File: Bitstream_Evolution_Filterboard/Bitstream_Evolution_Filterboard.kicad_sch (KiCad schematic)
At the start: 7 parts, among them J1 Conn_01x15_Female, J2 Conn_01x15_Female, J3 Conn_01x10_Female, J4 Conn_01x10_Female, J5 Conn_01x02_Male

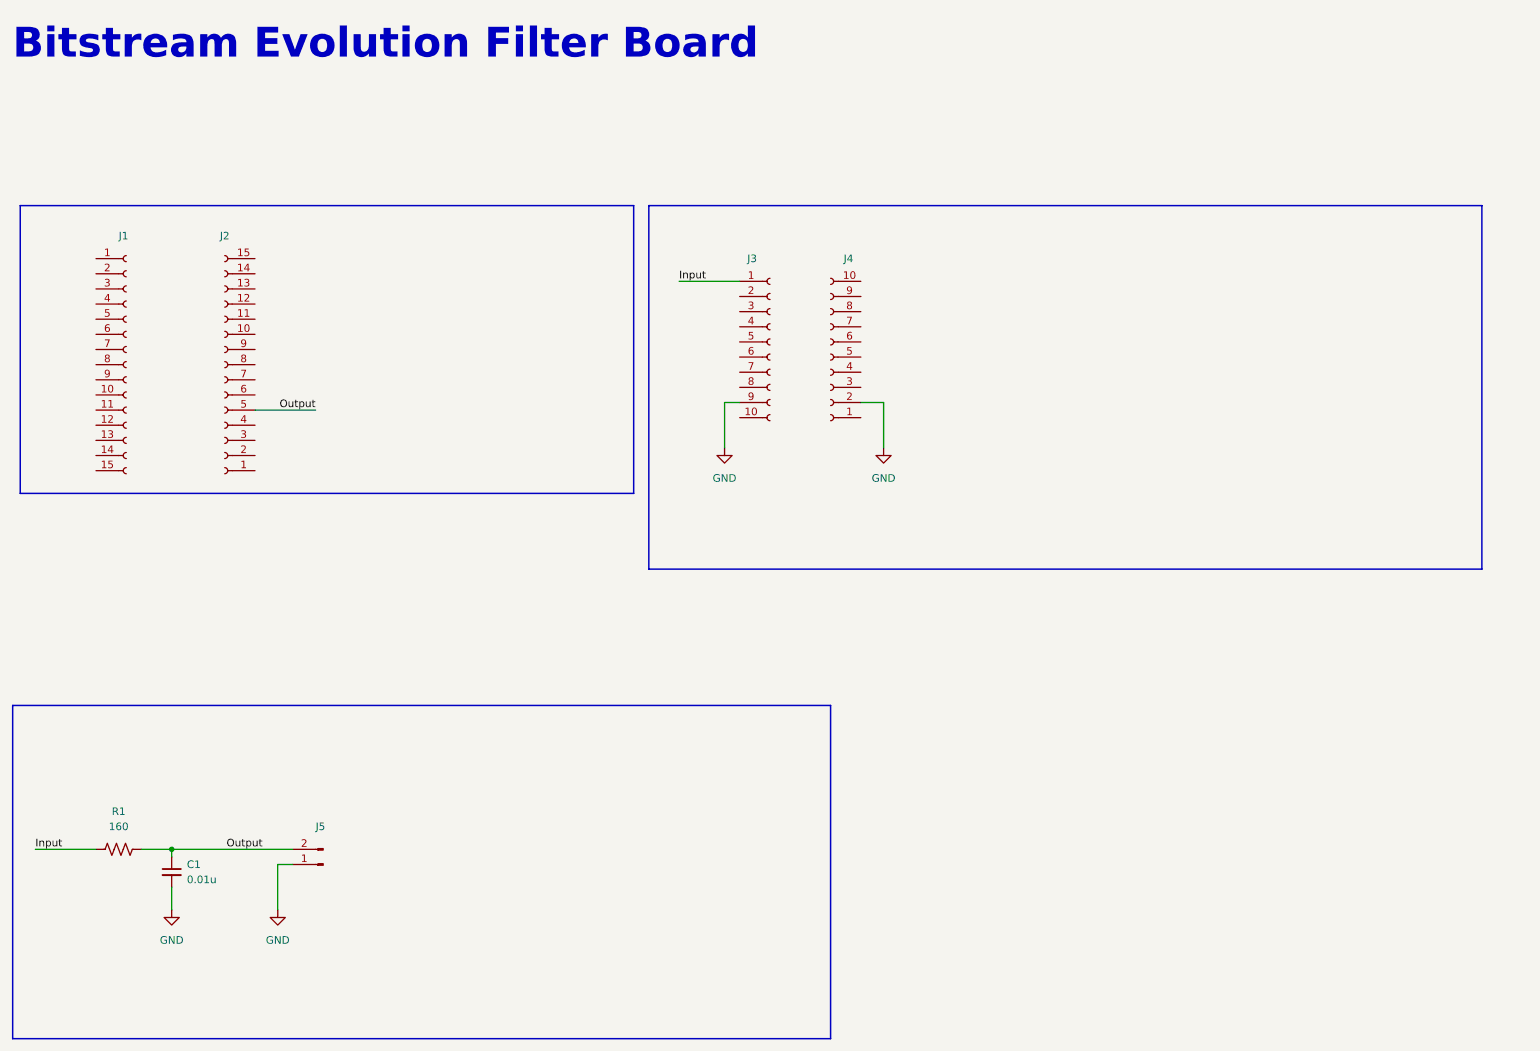
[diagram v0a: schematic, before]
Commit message: Updates to Hardware
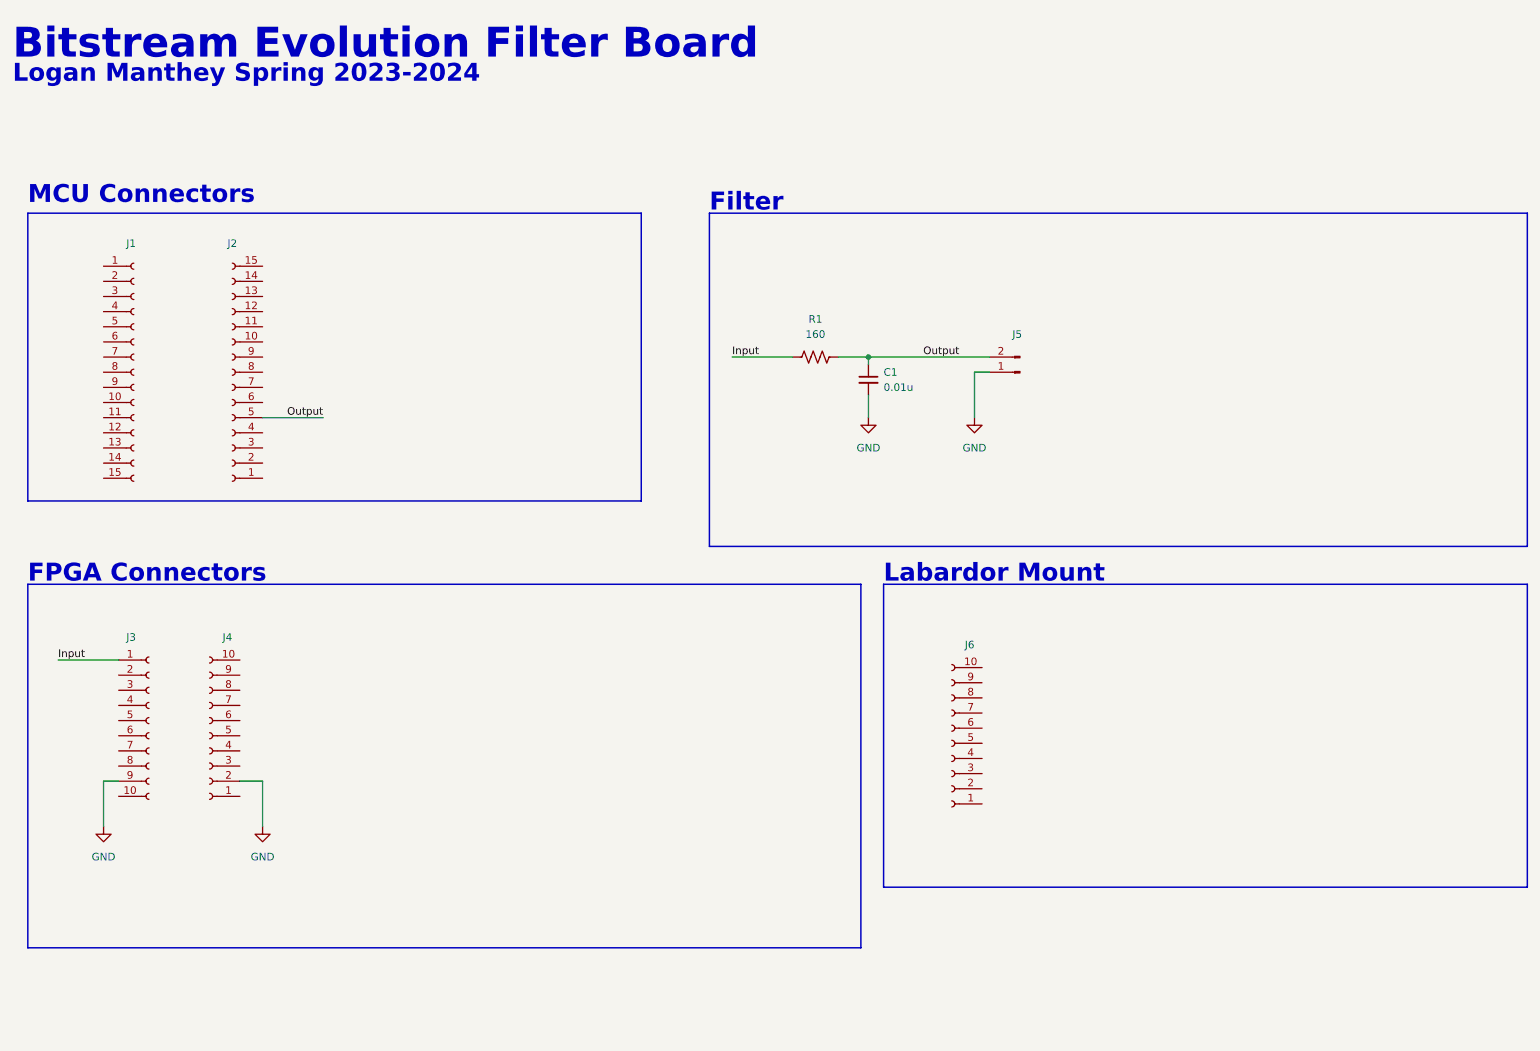
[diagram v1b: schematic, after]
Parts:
- added J6: Conn_01x10_Female, Connector_PinSocket_2.54mm:PinSocket_1x10_P2.54mm_Vertical, symbol Connector:Conn_01x10_Female
- J1, J2: footprint Connector_PinSocket_1.00mm:PinSocket_1x15_P1.00mm_Vertical -> Connector_PinSocket_2.54mm:PinSocket_1x15_P2.54mm_Vertical
- J3, J4: footprint Connector_PinSocket_1.00mm:PinSocket_1x10_P1.00mm_Vertical -> Connector_PinSocket_2.54mm:PinSocket_1x10_P2.54mm_Vertical
- J5: footprint Connector_PinHeader_2.00mm:PinHeader_1x02_P2.00mm_Vertical -> Connector_PinSocket_2.54mm:PinSocket_1x02_P2.54mm_Vertical
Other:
- note added: "FPGA Connectors"
- note added: "Filter"
- note added: "Labardor Mount"
- note added: "Logan Manthey Spring 2023-2024"
- note added: "MCU Connectors"
- moved on the sheet: C1, J1, J2, J3, J4, J5, R1
